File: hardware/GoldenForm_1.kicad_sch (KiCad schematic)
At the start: 56 parts, among them IC1 UVLO, J1 1140084168, J2 Conn_01x02_Pin, J3 USB4105-GF-A, J4 Conn_01x04_Pin, J5 Conn_01x02_Pin, M1 MountingHole x 4, U1 ESP32-S3-WROOM-1, U2 BNO055, U3 Buck_Boost, U4 AO3400A

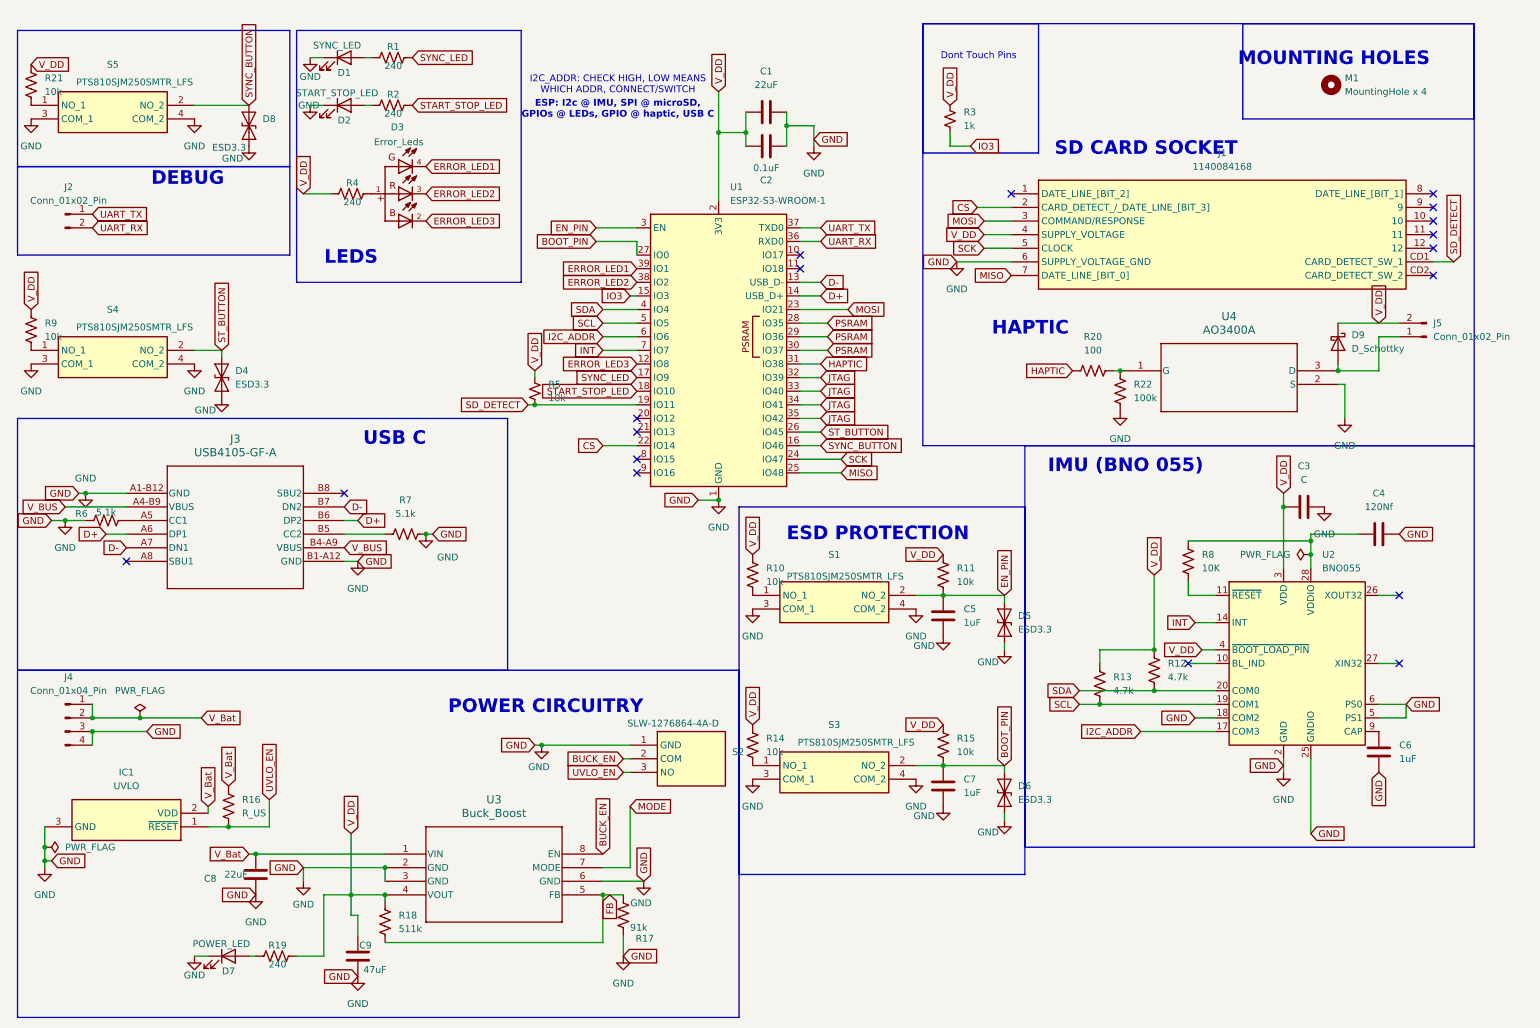
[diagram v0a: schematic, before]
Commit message: started routing. added classes and stuff
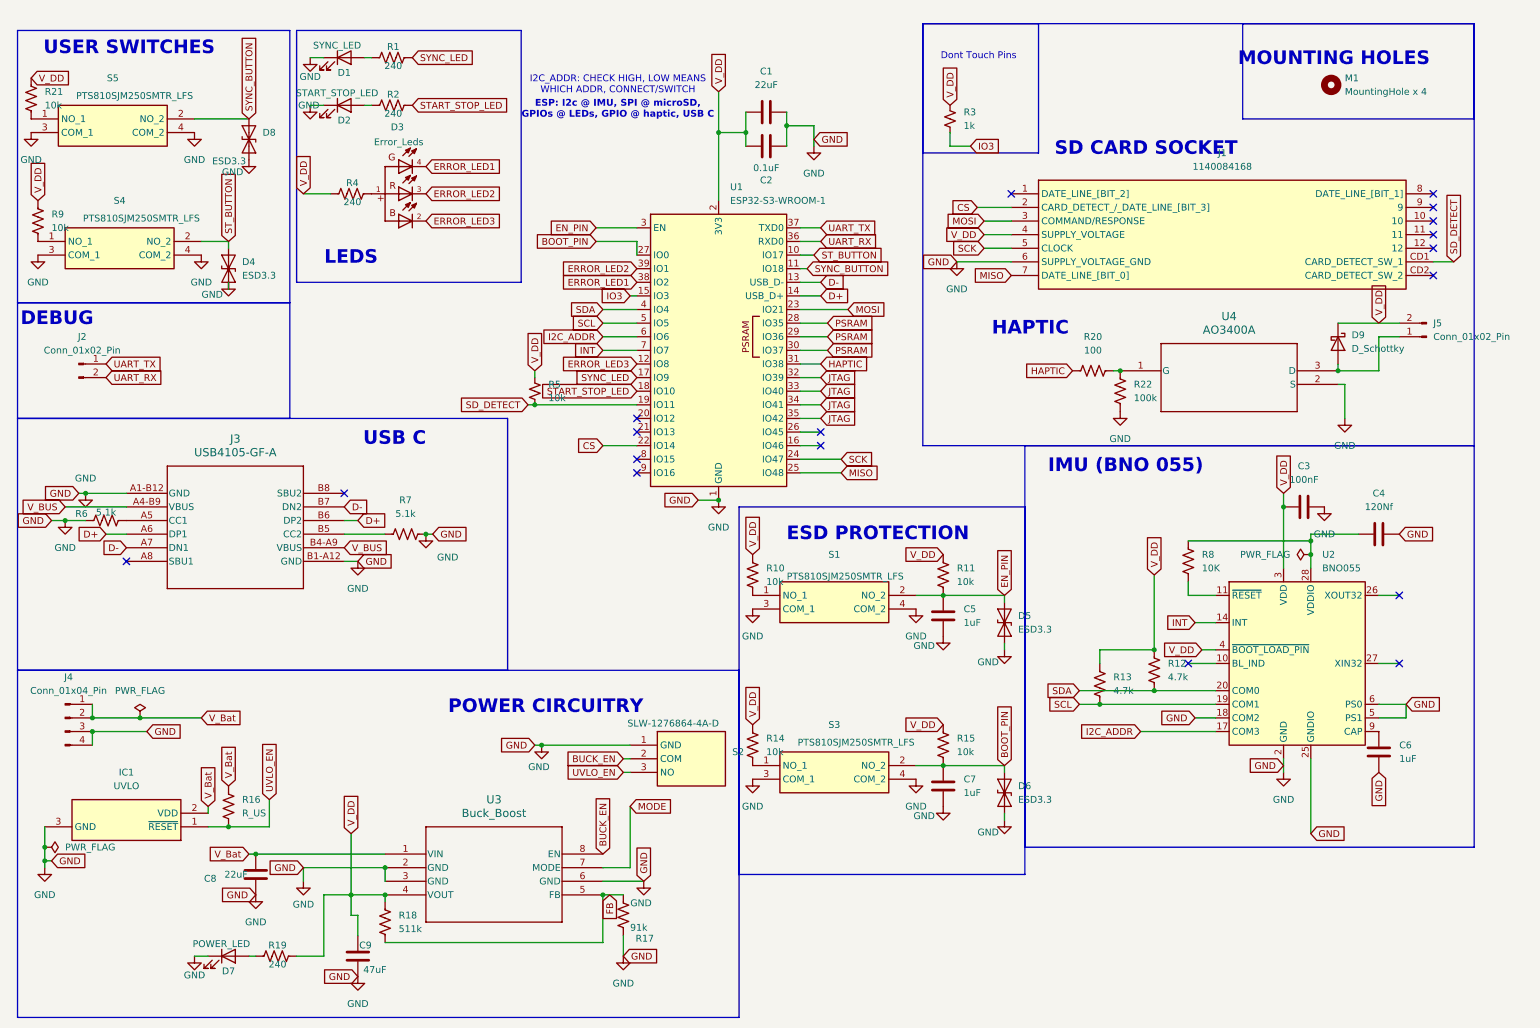
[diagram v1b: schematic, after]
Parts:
- C3: value C -> 100nF
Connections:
- net ERROR_LED1: now also U1.38 (IO2); no longer U1.39 (IO1)
- net ERROR_LED2: now also U1.39 (IO1); no longer U1.38 (IO2)
- net ST_BUTTON: now also U1.10 (IO17); no longer U1.26 (IO45)
- net SYNC_BUTTON: now also U1.11 (IO18); no longer U1.16 (IO46)
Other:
- note added: "USER SWITCHES"
- moved on the sheet: D4, D8, J2, R21, R9, S4, S5
